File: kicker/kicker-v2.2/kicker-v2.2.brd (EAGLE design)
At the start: 152.8 x 55 mm, 53 parts, among them IC1 7818TV, IC2 MCP601OT, J1 XT-60BATT_LABEL, Q1 IGB50N60T, Q3 IGB50N60T, U1 LT3750EMSPBF, U2 ATMEGA328P-AU

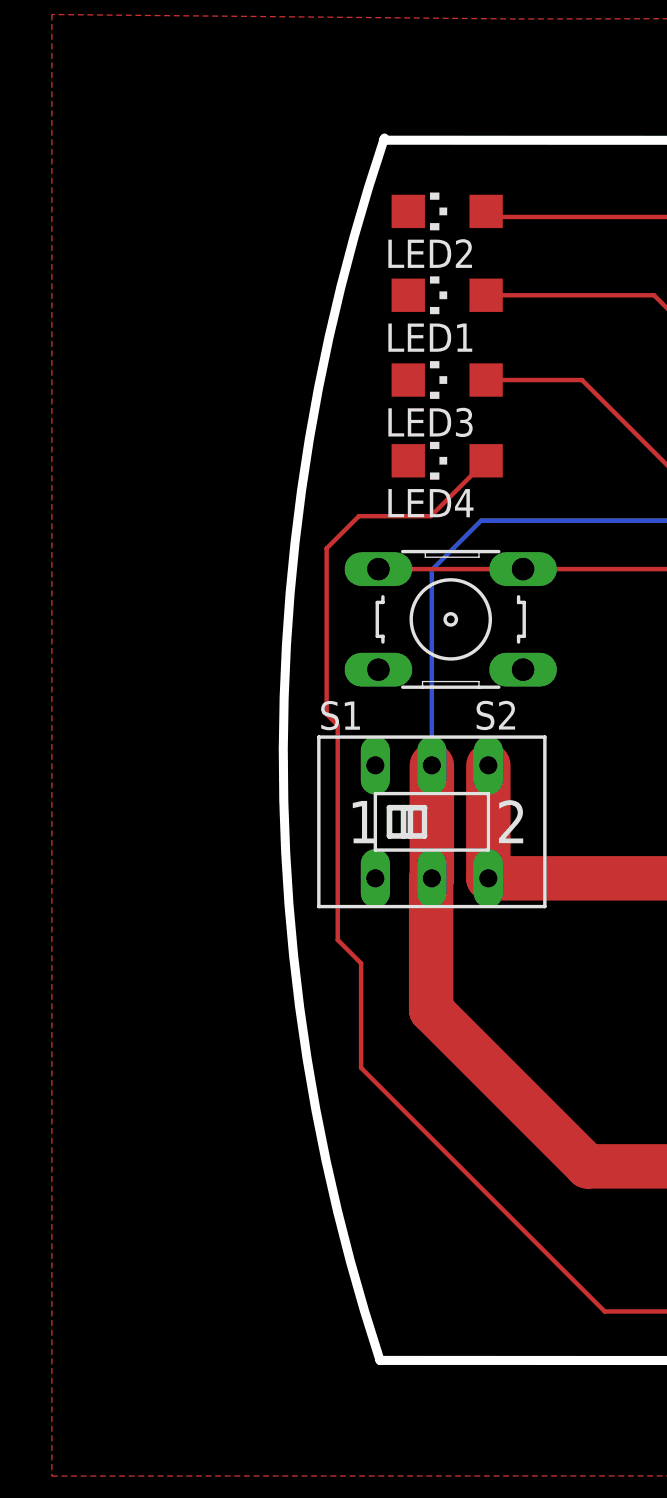
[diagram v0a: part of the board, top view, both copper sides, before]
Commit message: Enclosed Loop
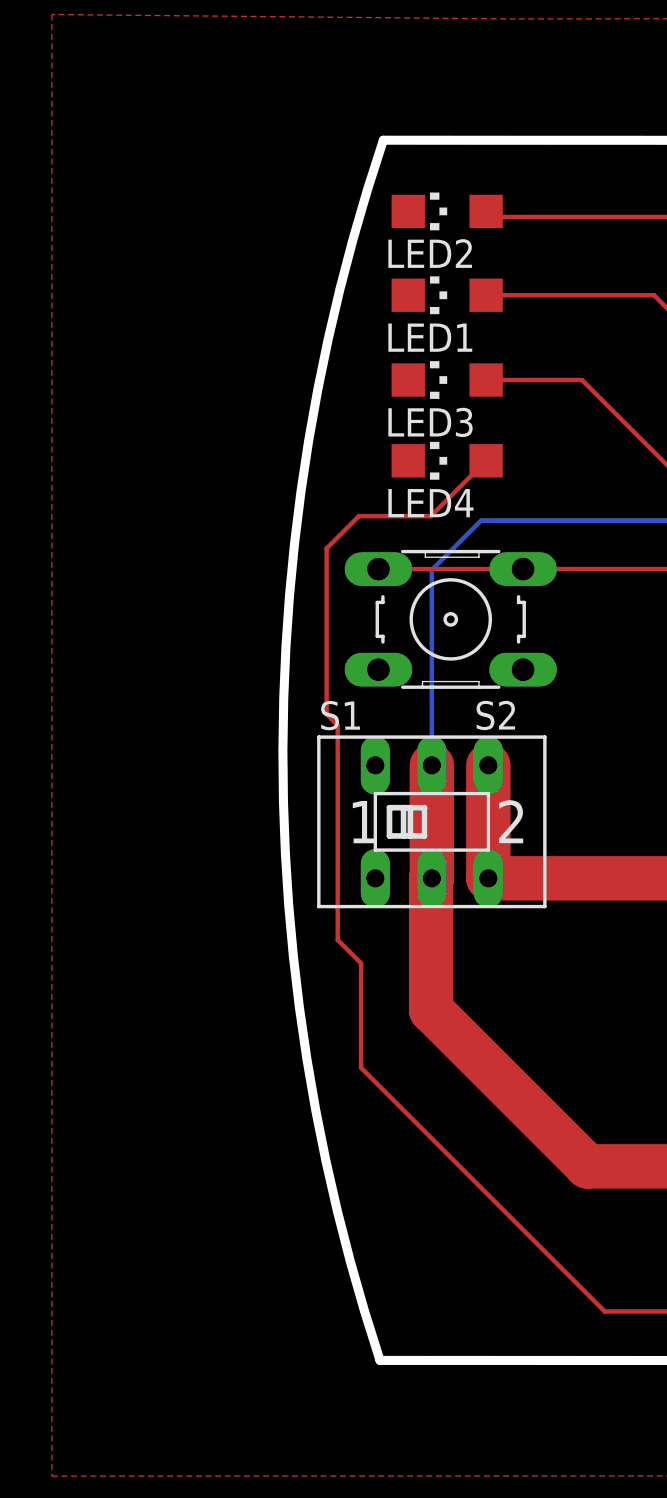
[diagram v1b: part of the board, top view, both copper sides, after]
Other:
- board size 152.8 x 55 mm -> 152.9 x 54.9 mm
